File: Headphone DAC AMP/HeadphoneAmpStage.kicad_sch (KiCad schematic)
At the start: 66 parts, among them U3 TPA6120A2DWP, U4 OPA1612AxD, U5 OPA1612AxD

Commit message: Schematic V1 Done
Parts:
- R11, R12: footprint Resistor_THT:R_Axial_DIN0207_L6.3mm_D2.5mm_P10.16mm_Horizontal -> Capacitor_SMD:C_0805_2012Metric_Pad1.18x1.45mm_HandSolder
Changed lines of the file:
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@@
 			"AAAAAAAAAAAAAAAAAAAAAAAAAAAAAAAAAAAAAAAAAAAAAAAAAAAAAAAAAAAAAAAAAAAAAAAAAAAA"
 			"AAAAAAAAAAAAAAAAAAAAAAAAAAAAAAAAAAAAAAAAAAAAAAAAAAAAAAAAAAAAAAAAAAAAAAAAAAAA"
+			"AAAAAAAAAAAAAAAAAAAAAAAAAAAAAAAAAAAAAAAAAAAAAAAAAAAAAAAAAAAAAAAAAAAAAAAAAAAA"
+			"AAAAAAAAAAAAAAAAAAAAAAAAAAAAAAAAAAAAAAAAAAAAAAAAAAAAAAAAAAAAAAAAAAAAAAAAAAAA"
+			"AAAAAAAAAAAAAAAAAAAAAAAAAAAAAAAAAAAAAAAAAAAAAAAAAAAAAAAAAAAAAAAAAAAAAAAAAAAA"
+			"AAAAAAAAAAAAAAAAAAAAAAAAAAAAAAAAAAAAAAAAAAAAAAAAAAAAAAAAAAAAAAAAAAAAAAAAAAAA"
+			"AAAAAAAAAAAAAAAAAAAAAAAAAAAAAAAAAAAAAAAAAAAAAAAAAAAAAAAAAAAAAAAAAAAAAAAAAAAA"
+			"AAAAAAAAAAAAAAAAAAAAAAAAAAAAAAAAAAAAAAAAAAAAAAAAAAAAAAAAAAAAAAAAAAAAAAAAAAAA"
+			"AAAAAAAAAAAAAAAAAAAAAAAAAAAAAAAAAAAAAAAAAAAAAAAAAAAAAAAAAAAAAAAAAAAAAAAAAAAA"
+			"AAAAAAAAAAAAAAAAAAAAAAAAAAAAAAAAAAAAAAAAAAAAAAAAAAAAAAAAAAAAAAAAAAAAAAAAAAAA"
+			"AAAAAAAAAAAAAAAAAAAAAAAAAAAAAAAAAAAAAAAAAAAAAAAAAAAAAAAAAAAAAAAAAAAAAAAAAAAA"
+			"AAAAAAAAAAAAAAAAAAAAAAAAAAAAAAAAAAAAAAAAAAAAAAAAAAAAAAAAAAAAAAAAAAAAAAAAAAAA"
+			"AAAAAAAAAAAAAAAAAAAAAAAAAAAAAAAAAAAAAAAAAAAAAAAAAAAAAAAAAAAAAAAAAAAAAAAAAAAA"
+			"AAAAAAAAAAAAAAAAAAAAAAAAAAAAAAAAAAAAAAAAAAAAAAAAAAAAAAAAAAAAAAAAAAAAAAAAAAAA"
+			"AAAAAAAAAAAAAAAAAAAAAAAAAAAAAAAAAAAAAAAAAAAAAAAAAAAAAAAAAAAAAAAAAAAAAAAAAAAA"
+			"AAAAAAAAAAAAAAAAAAAAAAAAAAAAAAAAAAAAAAAAAAAAAAAAAAAAAAAAAAAAAAAAAAAAAAAAAAAA"
+			"AAAAAAAAAAAAAAAAAAAAAAAAAAAAAAAAAAAAAAAAAAAAAAAAAAAAAAAAAAAAAAAAAAAAAAAAAAAA"
+			"AAAAAAAAAAAAAAAAAAAAAAAAAAAAAAAAAAAAAAAAAAAAAAAAAAAAAAAAAAAAAAAAAAAAAAAAAAAA"
+			"AAAAAAAAAAAAAAAAAAAAAAAAAAAAAAAAAAAAAAAAAAAAAAAAAAAAAAAAAAAAAAAAAAAAAAAAAAAA"
+			"AAAAAAAAAAAAAAAAAAAAAAAAAAAAAAAAAAAAAAAAAAAAAAAAAAAAAAAAAAAAAAAAAAAAAAAAAAAA"
 			"AAAAAAAAAAAAAAAAAAAAAAAAAAAAAAAAAAAAAAAAAAAAAAAAAA=="
 		)
@@
 		(exclude_from_sim no)
 		(in_bom yes)
-		(on_board yes)
+		(on_board no)
 		(dnp no)
 		(fields_autoplaced yes)
@@
 			)
 		)
-		(property "Footprint" "Resistor_THT:R_Axial_DIN0207_L6.3mm_D2.5mm_P10.16mm_Horizontal"
+		(property "Footprint" "Capacitor_SMD:C_0805_2012Metric_Pad1.18x1.45mm_HandSolder"
 			(at 156.591 24.892 0)
 			(effects
@@
 		(exclude_from_sim no)
 		(in_bom yes)
-		(on_board yes)
+		(on_board no)
 		(dnp no)
 		(fields_autoplaced yes)
@@
 			)
 		)
-		(property "Footprint" "Resistor_THT:R_Axial_DIN0207_L6.3mm_D2.5mm_P10.16mm_Horizontal"
+		(property "Footprint" "Capacitor_SMD:C_0805_2012Metric_Pad1.18x1.45mm_HandSolder"
 			(at 255.651 27.432 0)
 			(effects

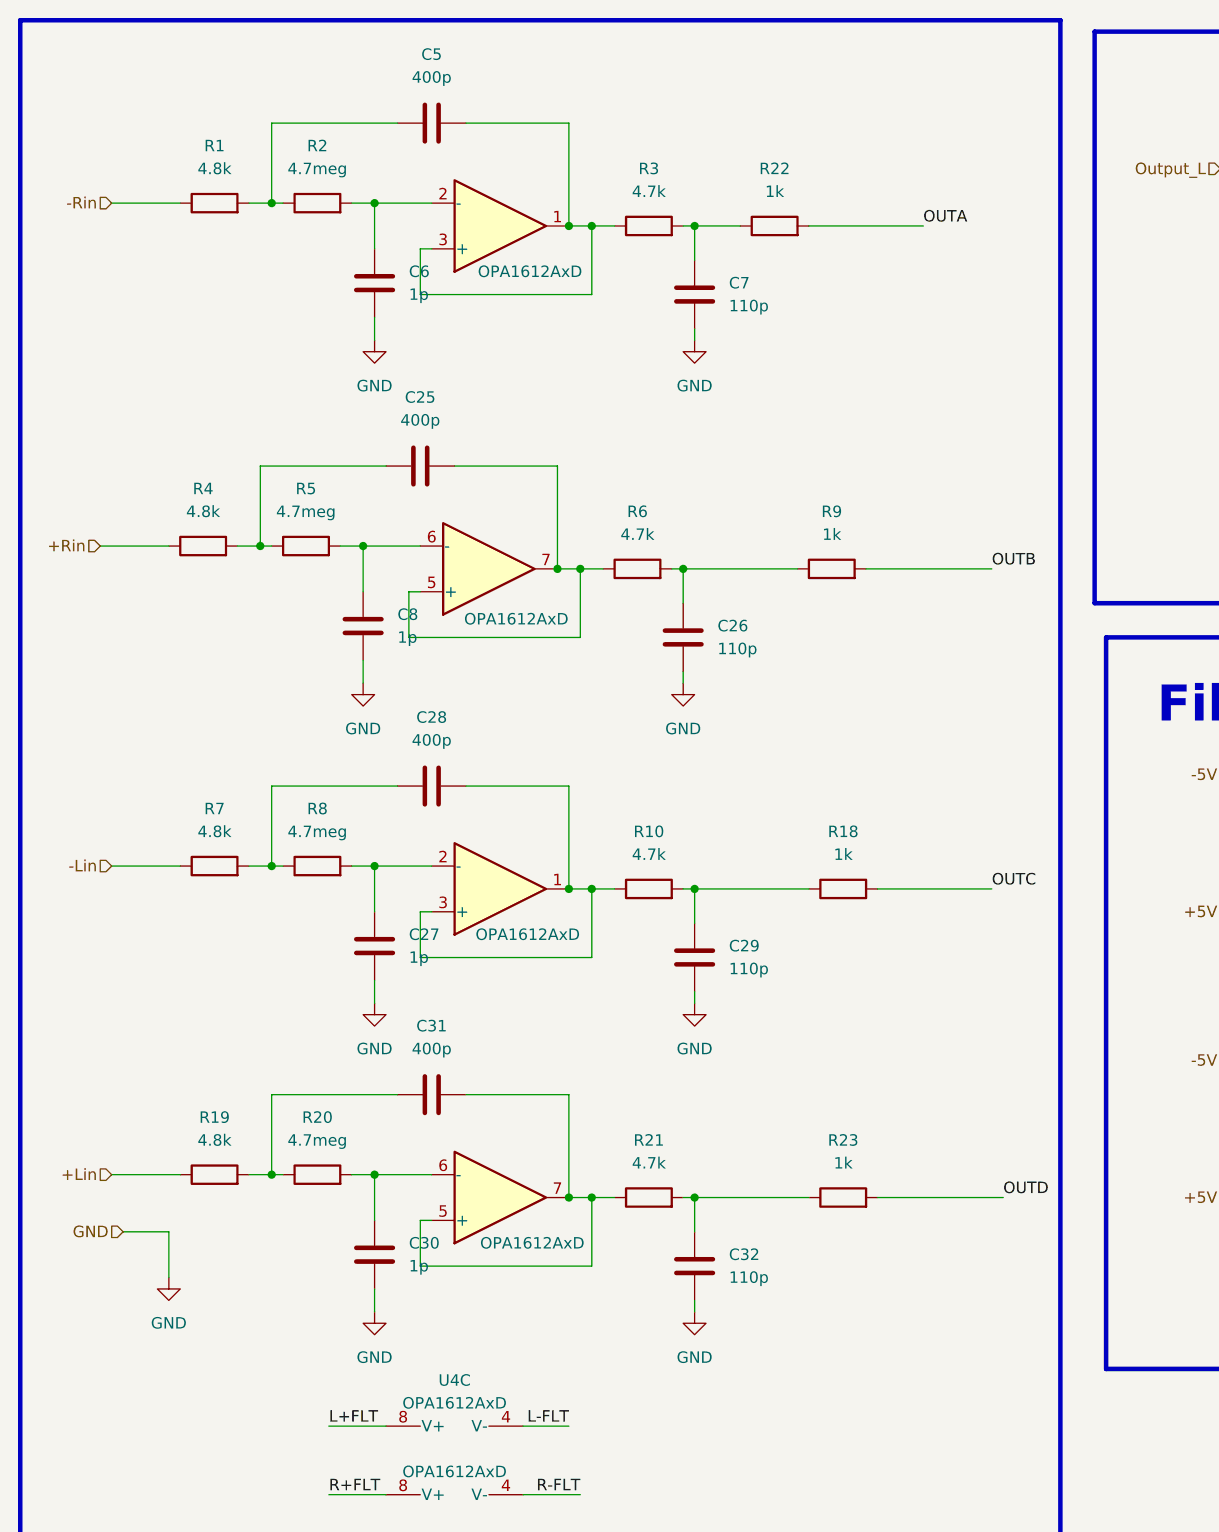
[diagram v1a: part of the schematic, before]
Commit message: Fixed all the work i put in
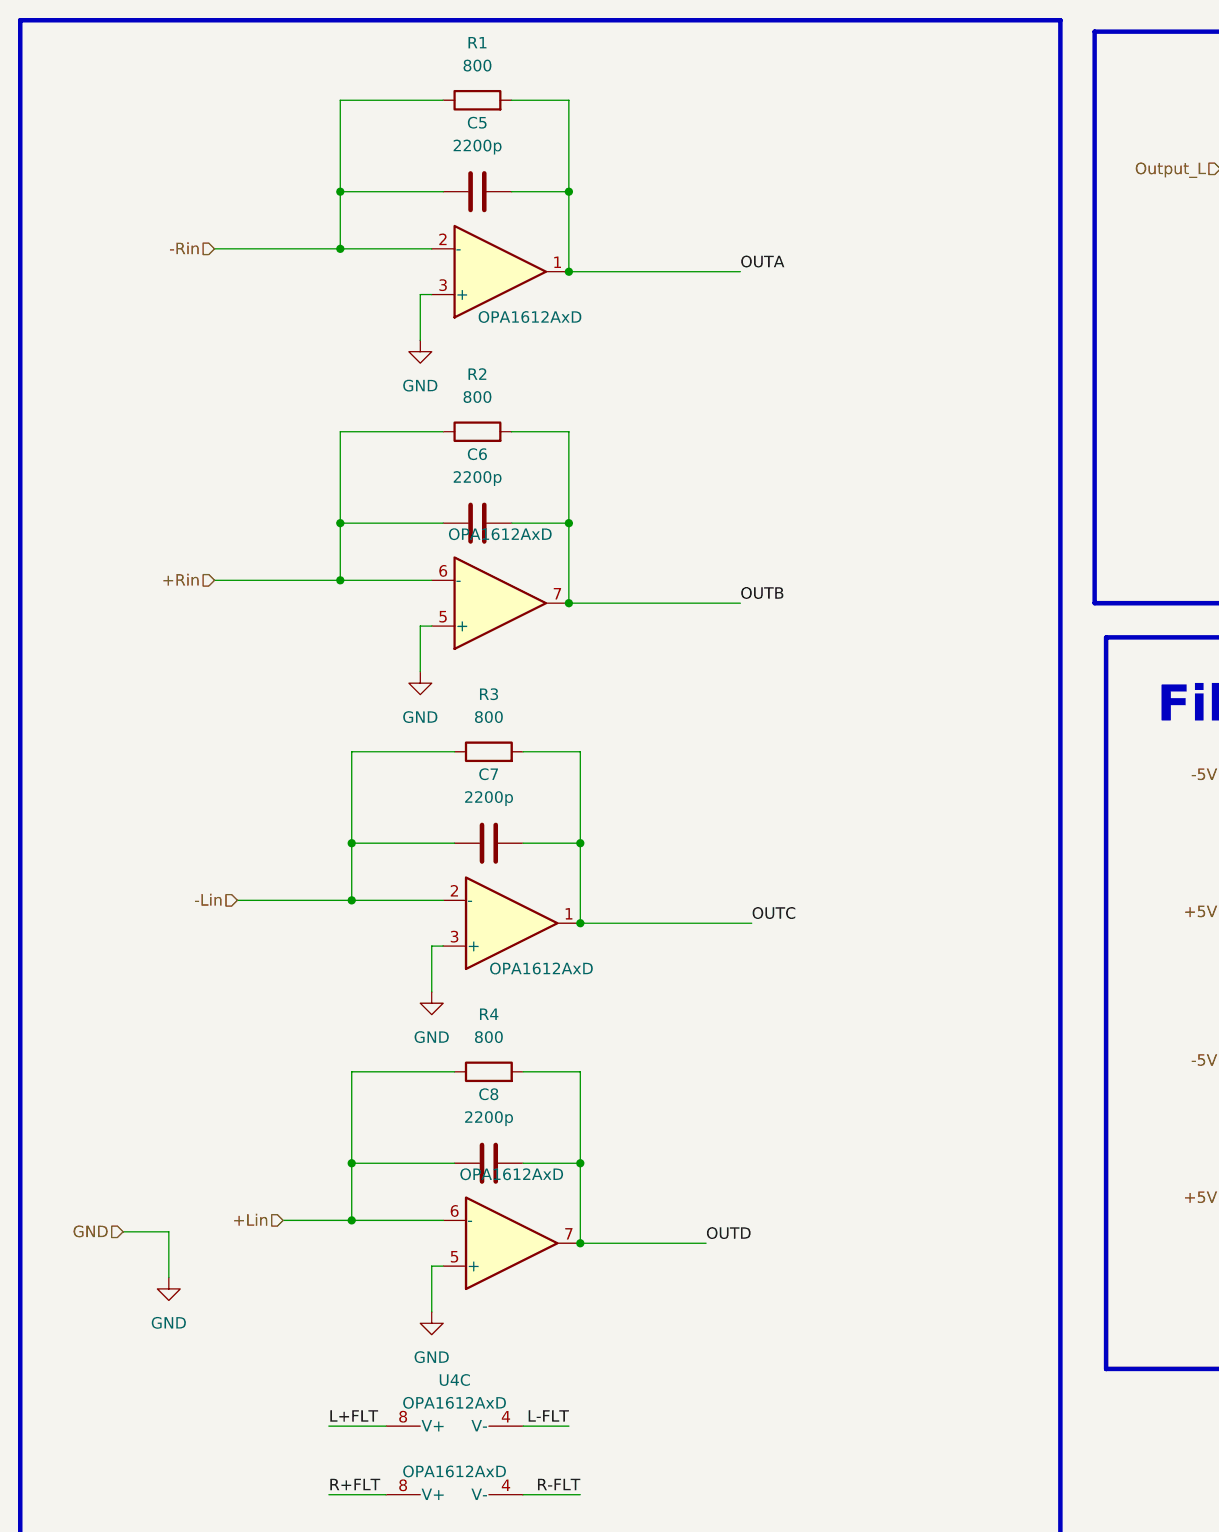
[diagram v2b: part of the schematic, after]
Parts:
- removed C25, C28, C31: 400p, Capacitor_SMD:C_0805_2012Metric_Pad1.18x1.45mm_HandSolder, symbol Device:C
- removed C26, C29, C32: 110p, Capacitor_SMD:C_0805_2012Metric_Pad1.18x1.45mm_HandSolder, symbol Device:C
- removed C27, C30: 1p, Capacitor_SMD:C_0805_2012Metric_Pad1.18x1.45mm_HandSolder, symbol Device:C
- removed R10, R21, R6: 4.7k, Resistor_SMD:R_0805_2012Metric_Pad1.20x1.40mm_HandSolder, symbol Device:R
- removed R18, R22, R23, R9: 1k, Resistor_SMD:R_0805_2012Metric_Pad1.20x1.40mm_HandSolder, symbol Device:R
- removed R19, R7: 4.8k, Resistor_SMD:R_0805_2012Metric_Pad1.20x1.40mm_HandSolder, symbol Device:R
- removed R20, R5, R8: 4.7meg, Resistor_SMD:R_0805_2012Metric_Pad1.20x1.40mm_HandSolder, symbol Device:R
- removed unit 2 of U4
- removed unit 2 of U5
- C5: value 400p -> 2200p
- C6, C8: value 1p -> 2200p
- C7: value 110p -> 2200p
- R1, R4: value 4.8k -> 800
- R2: value 4.7meg -> 800
- R3: value 4.7k -> 800
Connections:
- net +Lin: now also C8.1, R4.1, U5.6 (-)
- net +Rin: now also C6.1, R2.1, U4.6 (-); no longer R4.1
- net -Lin: now also C7.1, R3.1, U5.2 (-)
- net -Rin: now also C5.1, U4.2 (-)
- net GND: now also U4.3 (+), U4.5 (+), U5.3 (+), U5.5 (+); no longer C6.2, C7.2, C8.2
- net OUTA: now also C5.2, R1.2, U4.1
- net OUTB: now also C6.2, R2.2, U4.7
- net OUTC: now also C7.2, R3.2, U5.1
- net OUTD: now also C8.2, R4.2, U5.7
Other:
- moved on the sheet: C5, R1
